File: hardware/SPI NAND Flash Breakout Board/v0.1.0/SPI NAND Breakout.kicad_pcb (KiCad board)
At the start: 2 copper layers, 32 x 24 mm, 14 parts, among them J1 Conn_01x08_Pin, U1 AS5F18G04SND-10LIN, U2 TXB0106PW, U3 AP2127K-1.8

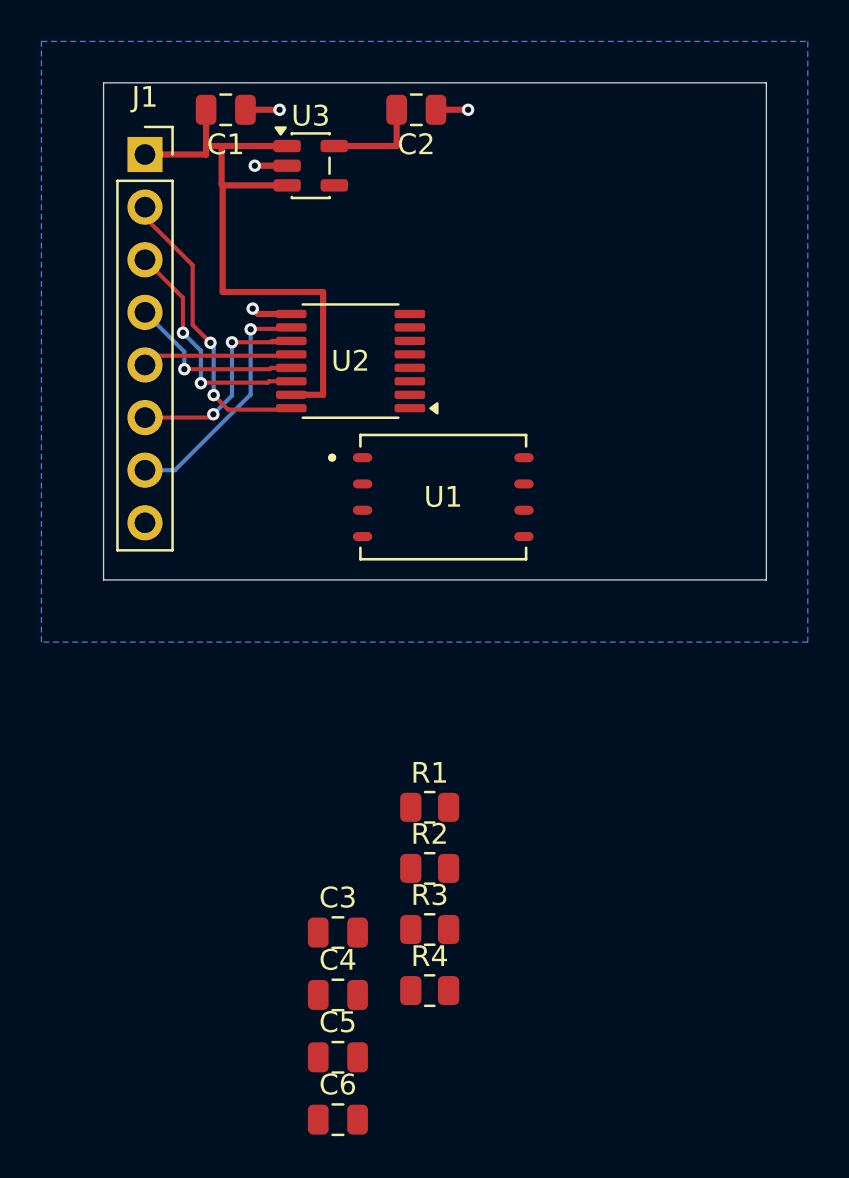
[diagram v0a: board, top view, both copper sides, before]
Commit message: gbr files
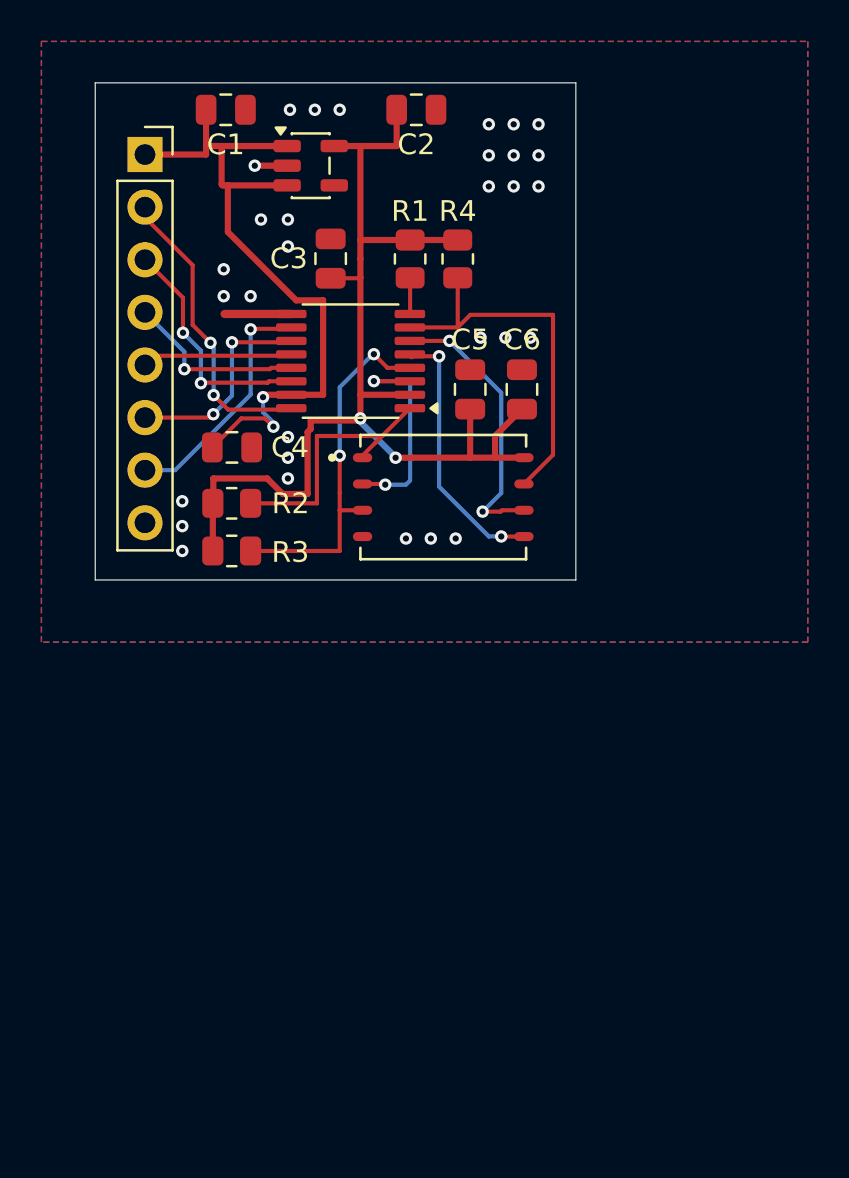
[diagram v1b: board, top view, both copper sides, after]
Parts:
- moved C6 36.4 mm to (170.2, 91.8), turned to 90 degrees
- moved R4 35.4 mm to (167.1, 85.5), turned to -90 degrees
- moved C5 32.9 mm to (167.7, 91.8), turned to 90 degrees
- moved C3 32.5 mm to (161.0, 85.5), turned to -90 degrees
- moved C4 26.9 mm to (156.2, 94.6), turned to 180 degrees
- moved R1 26.5 mm to (164.8, 85.5), turned to -90 degrees
- moved R3 20.6 mm to (156.2, 99.6)
- moved R2 20.0 mm to (156.2, 97.3), turned to 180 degrees
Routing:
- net Net-(U1-VCC): track 4.76 -> 54.9 mm, vias 0 -> 2
- net Net-(U1-HOLD#/SIO3): track 0.00 -> 18.3 mm
- net Net-(U1-WP#/SIO2): track 0.00 -> 17.7 mm, vias 0 -> 2
- net Net-(U1-SCLK): track 0.00 -> 13.6 mm, vias 0 -> 2
- net Net-(U1-CS#): track 0.00 -> 12.9 mm
- net Net-(U1-SI/SIO0): track 0.00 -> 12.8 mm, vias 0 -> 2
- net Net-(U1-SO/SIO1): track 0.00 -> 10.7 mm, vias 0 -> 2
- net Net-(J1-Pin_1): track 30.6 -> 35.1 mm, vias 0 -> 2
- net GND: track 6.73 -> 4.84 mm, vias 4 -> 31
- net Net-(U2-OE): track 0.00 -> 1.75 mm
- net Net-(J1-Pin_6): track 11.2 -> 10.2 mm
- added copper zone on F.Cu, net GND
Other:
- board size 32 x 24 mm -> 23.2 x 24 mm
- board text added: "3.3V"
- board text added: "CS#"
- board text added: "Flash: AS5F18G04SND-10LIN"
- board text added: "GND"
- board text added: "HOLD#/IO 3"
- board text added: "IO 0"
- board text added: "IO 1"
- board text added: "SCLK"
- board text added: "WP#/IO 2"
